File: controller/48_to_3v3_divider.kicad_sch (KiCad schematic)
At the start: 5 parts

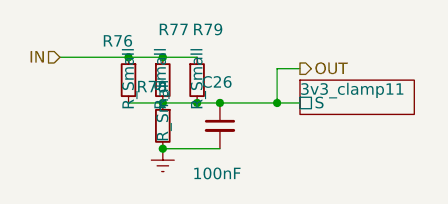
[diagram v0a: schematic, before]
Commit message: Controller - Try to simplify
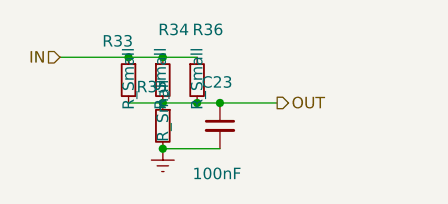
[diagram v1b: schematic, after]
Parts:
- renumbered C26 to C23, R76 to R33, R77 to R34, R78 to R35, R79 to R36
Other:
- removed sheet 3v3_clamp11
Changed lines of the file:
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@@
-	)
-	(junction
-		(at 44.45 30.48)
-		(diameter 0)
-		(color 0 0 0 0)
 	)
 	(junction
@@
 	(wire
 		(pts
-			(xy 44.45 26.67) (xy 44.45 30.48)
-		)
-		(stroke
-			(width 0)
-			(type default)
-		)
-	)
-	(wire
-		(pts
-			(xy 44.45 30.48) (xy 46.99 30.48)
-		)
-		(stroke
-			(width 0)
-			(type default)
-		)
-	)
-	(wire
-		(pts
-			(xy 46.99 26.67) (xy 44.45 26.67)
-		)
-		(stroke
-			(width 0)
-			(type default)
-		)
-	)
-	(wire
-		(pts
 			(xy 35.56 30.48) (xy 38.1 30.48)
 		)
@@
 	(hierarchical_label "OUT"
 		(shape output)
-		(at 46.99 26.67 0)
+		(at 44.45 30.48 0)
 		(fields_autoplaced yes)
 		(effects
@@
 		(on_board yes)
 		(dnp no)
-		(property "Reference" "R77"
+		(property "Reference" "R34"
 			(at 31.242 22.352 0)
 			(effects
@@
 		(on_board yes)
 		(dnp no)
-		(property "Reference" "R79"
+		(property "Reference" "R36"
 			(at 35.052 22.352 0)
 			(effects
@@
 		(on_board yes)
 		(dnp no)
-		(property "Reference" "R78"
+		(property "Reference" "R35"
 			(at 32.258 28.702 0)
 			(effects
@@
 		(dnp no)
 		(fields_autoplaced yes)
-		(property "Reference" "#PWR090"
+		(property "Reference" "#PWR053"
 			(at 31.75 41.91 0)
 			(effects
@@
 		(on_board yes)
 		(dnp no)
-		(property "Reference" "R76"
+		(property "Reference" "R33"
 			(at 28.448 23.622 0)
 			(effects
@@
 		(on_board yes)
 		(dnp no)
-		(property "Reference" "C26"
+		(property "Reference" "C23"
 			(at 36.068 28.194 0)
 			(effects
@@
 				)
 			)
-		)
-	)
-	(sheet
-		(at 46.99 27.94)
-		(size 12.7 3.81)
-		(stroke
-			(width 0.1524)
-			(type solid)
-		)
-		(fill
-			(color 0 0 0 0.0000)
-		)
-		(property "Sheetname" "3v3_clamp11"
-			(at 46.99 29.718 0)
-			(effects
-				(font
-					(size 1.27 1.27)
-				)
-				(justify left bottom)
-			)
-		)
-		(property "Sheetfile" "mcu_clamp.kicad_sch"
-			(at 46.99 32.3346 0)
-			(effects
-				(font
-					(size 1.27 1.27)
-				)
-				(justify left top)
-				(hide yes)
-			)
-		)
-		(pin "S" passive
-			(at 46.99 30.48 180)
-			(effects
-				(font
-					(size 1.27 1.27)
-				)
-				(justify left)
-			)
-		)
-		(instances
-			(project "controller"
-				(path "/5b092a03-7e3e-4df1-ad91-2ac0e362f857/3a11ce7c-7e29-4758-a12a-8535ab4c73af"
-					(page "2")
-				)
-				(path "/5b092a03-7e3e-4df1-ad91-2ac0e362f857/8b76543b-a49c-413b-a98c-7f3e228c6216"
-					(page "4")
-				)
-				(path "/5b092a03-7e3e-4df1-ad91-2ac0e362f857/a5d84eb1-8829-4f32-a763-e01f5977372c"
-					(page "13")
-				)
-				(path "/5b092a03-7e3e-4df1-ad91-2ac0e362f857/2f911ebd-6dc8-4496-8afb-4a9ec6bafab7"
-					(page "15")
-				)
-				(path "/5b092a03-7e3e-4df1-ad91-2ac0e362f857/dfe157ff-eae8-44d0-adc3-b7fe75c1e740"
-					(page "17")
-				)
-				(path "/5b092a03-7e3e-4df1-ad91-2ac0e362f857/e3d09b0d-badf-46a0-b7fb-f25da99c9c12"
-					(page "19")
-				)
-			)

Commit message: Controller - More work mainly on layout
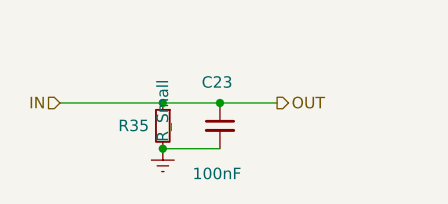
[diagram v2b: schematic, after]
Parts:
- removed R33, R34, R36: R_Small, Resistor_SMD:R_0805_2012Metric, symbol Device:R_Small
- C23: footprint Capacitor_SMD:C_0402_1005Metric -> Capacitor_SMD:C_0402_1005Metric_Pad0.74x0.62mm_HandSolder
- R35: footprint Resistor_SMD:R_0603_1608Metric -> Resistor_SMD:R_0402_1005Metric_Pad0.72x0.64mm_HandSolder
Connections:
- net OUT is gone; now on net IN: C23.1, R35.1
